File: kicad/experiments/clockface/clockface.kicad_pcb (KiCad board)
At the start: 2 copper layers, 50 x 50 mm, 11 parts, among them P1 CONN_01X05, U1 TOUCH_PAD_13, U2 MTCH6102_SSOP

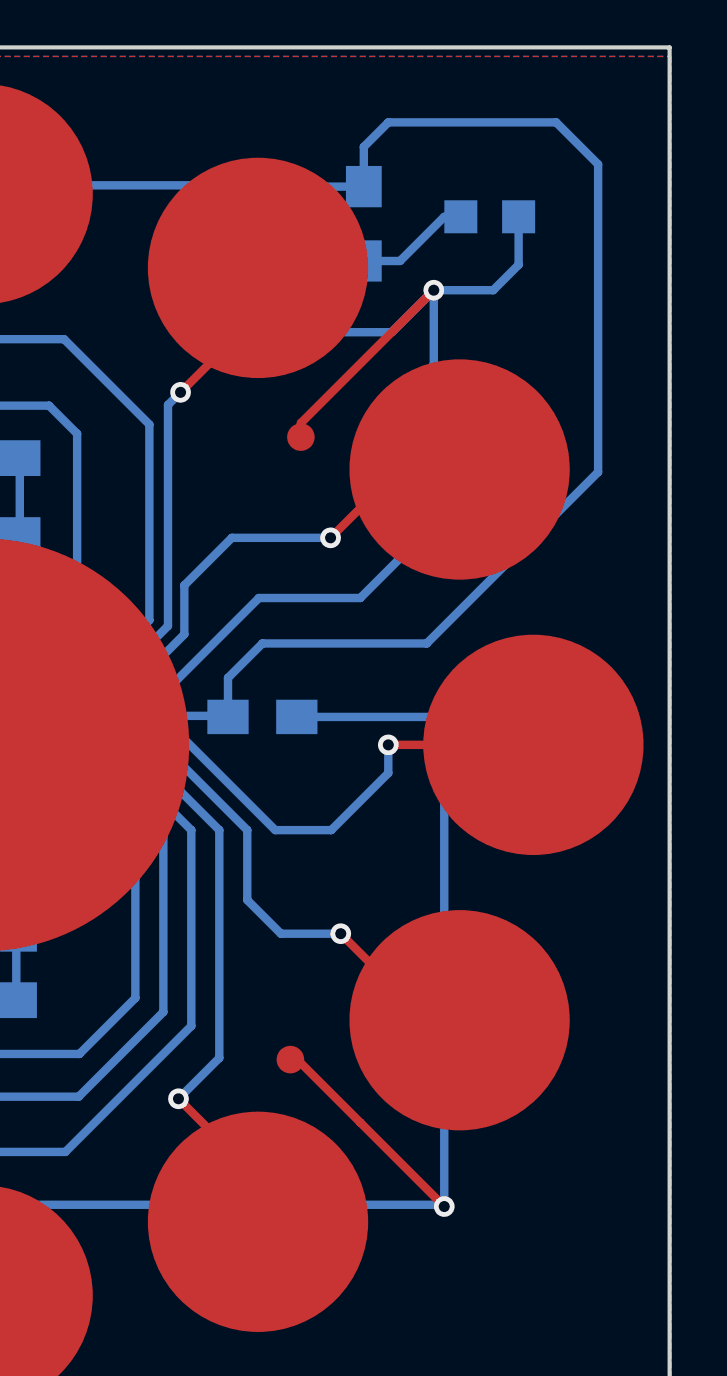
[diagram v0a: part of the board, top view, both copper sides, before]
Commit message: tweaks
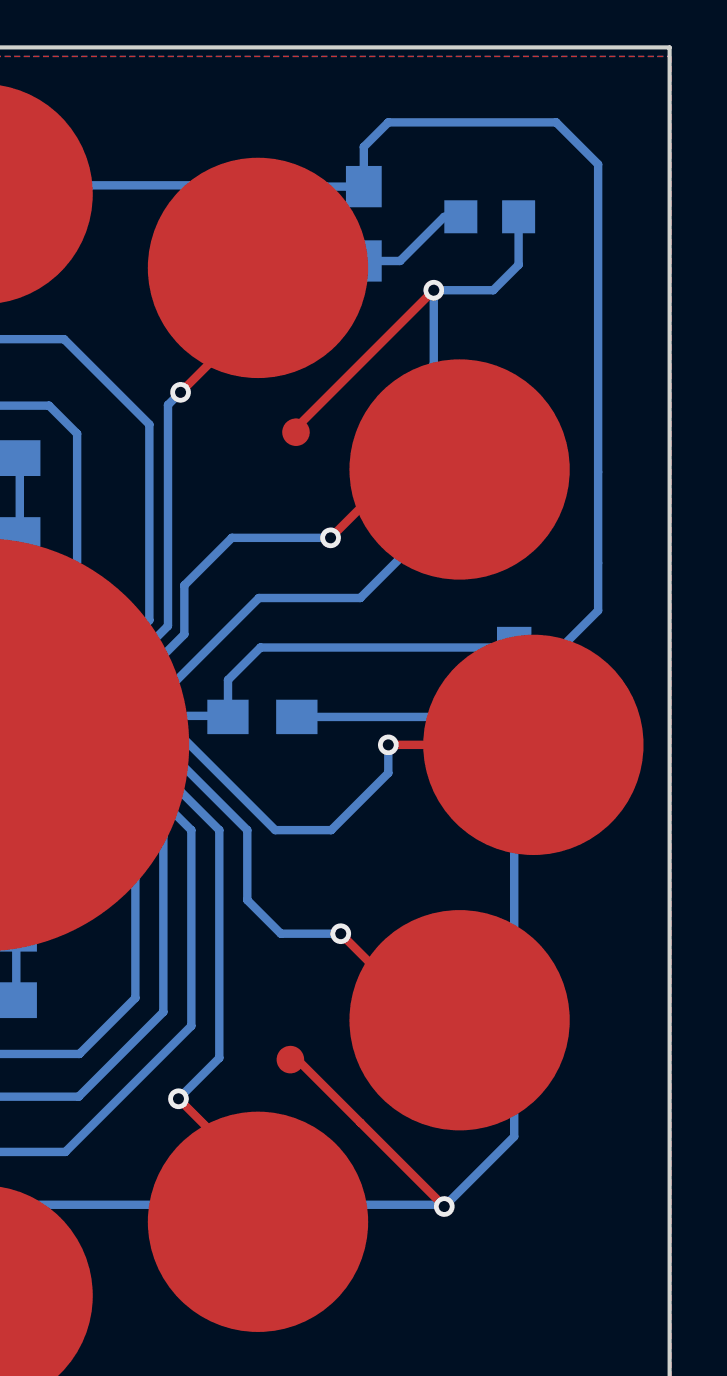
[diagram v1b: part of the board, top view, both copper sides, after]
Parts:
- moved C2 18.9 mm to (167.2, 91.6)
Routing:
- net GND: track 224.3 -> 219.7 mm
- net /3V3: track 91.9 -> 94.8 mm
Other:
- board text added: "https://github.com/theapi/touch_timer kicad/experiments/clockface v1.0"
